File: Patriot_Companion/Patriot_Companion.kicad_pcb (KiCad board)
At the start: 2 copper layers, 82 parts, among them P1 USB_OTG, P2 POWER_IN, P3 I/O, P4 CONN_02X03, P5 MOTOR_1, P6 MOTOR_2, P7 SERVO_HEADER, Q1 FDN340P, SW1 SWITCH, SW2 SWITCH, SW3 SWITCH, U1 LM358, U2 ATMEGA32U4-A, U3 LP2985-33DBVR, U4 7805, U5 BD6212HFP-TR, U6 NXP_MMA8652FCR1, U7 BD6212HFP-TR, U8 Si7006, Y1 16M

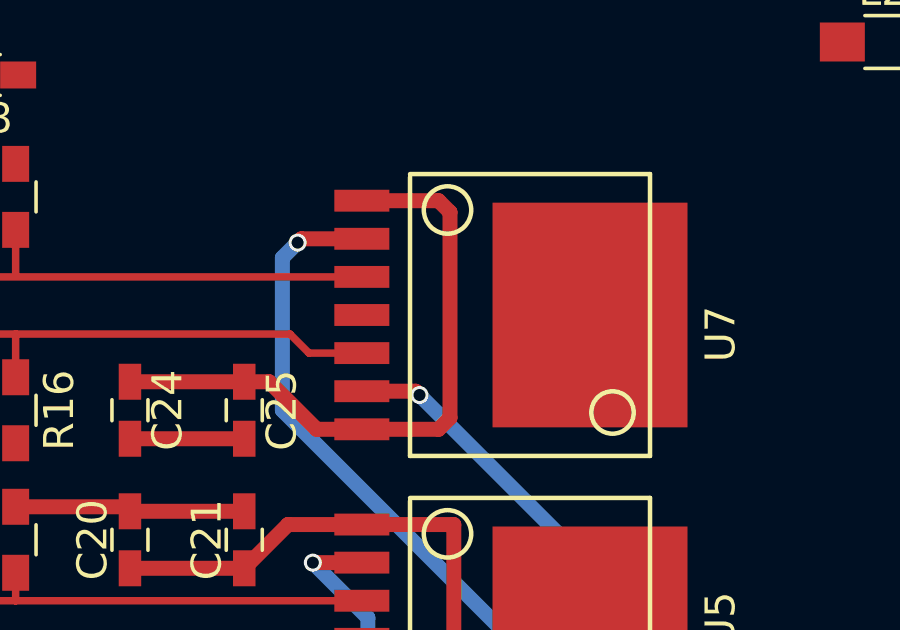
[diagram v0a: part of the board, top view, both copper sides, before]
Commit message: update
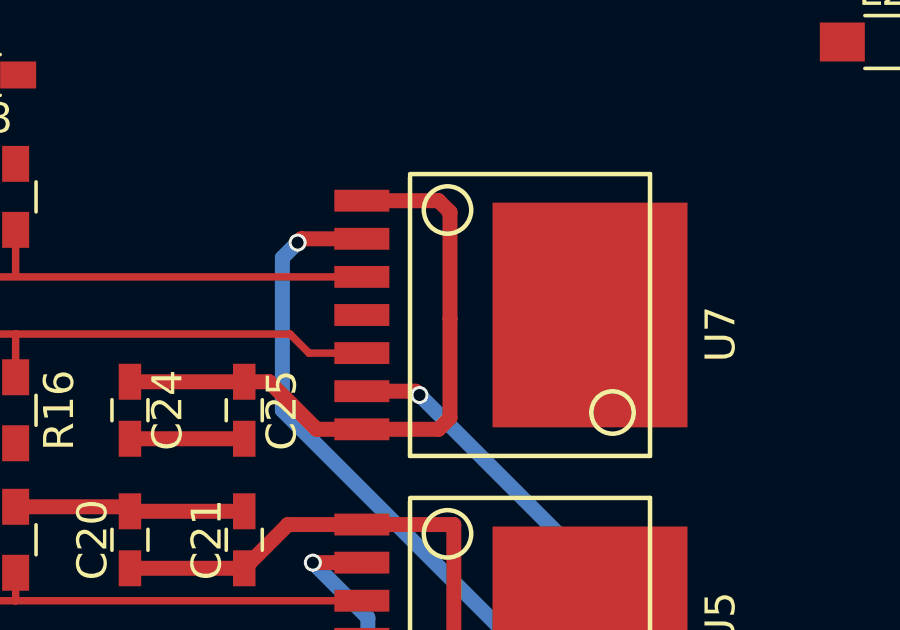
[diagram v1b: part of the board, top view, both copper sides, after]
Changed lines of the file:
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@@
     (links 203)
     (no_connects 183)
-    (area 34.801999 13.364999 229.409048 168.365)
+    (area 70.723 74.264 183.531001 171.451001)
     (thickness 1.6)
     (drawings 0)
-    (tracks 60)
+    (tracks 61)
     (zones 0)
     (modules 82)
@@
   (segment (start 124.31 137.838) (end 124.46 137.988) (width 0.5) (layer F.Cu) (net 2))
   (segment (start 124.46 137.988) (end 128.27 137.988) (width 0.5) (layer F.Cu) (net 2))
+  (segment (start 135.128 131.572) (end 135.128 134.874) (width 0.5) (layer F.Cu) (net 10))
+  (segment (start 135.128 128.016) (end 135.128 131.572) (width 0.5) (layer F.Cu) (net 10))
   (segment (start 132.1895 127.635) (end 134.747 127.635) (width 0.5) (layer F.Cu) (net 10))
   (segment (start 134.747 135.255) (end 132.1895 135.255) (width 0.5) (layer F.Cu) (net 10))
   (segment (start 135.128 134.874) (end 134.747 135.255) (width 0.5) (layer F.Cu) (net 10))
-  (segment (start 135.128 128.016) (end 135.128 134.874) (width 0.5) (layer F.Cu) (net 10))
   (segment (start 134.747 127.635) (end 135.128 128.016) (width 0.5) (layer F.Cu) (net 10))
   (segment (start 124.46 133.67) (end 128.27 133.67) (width 0.5) (layer F.Cu) (net 10))
